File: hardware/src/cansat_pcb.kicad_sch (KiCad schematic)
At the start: 9 parts, among them J1 Servo_motor, J2 Sen057_pressure_sensor, SW1 SPDT_Slide_SMD_6.7x2.6mm, U1 XIAO-nRF52840-Plus-SMD, U2 5V_booster, U3 Hall-effect_sensor, U4 BME280_sensor, U5 Openlog_SDcard

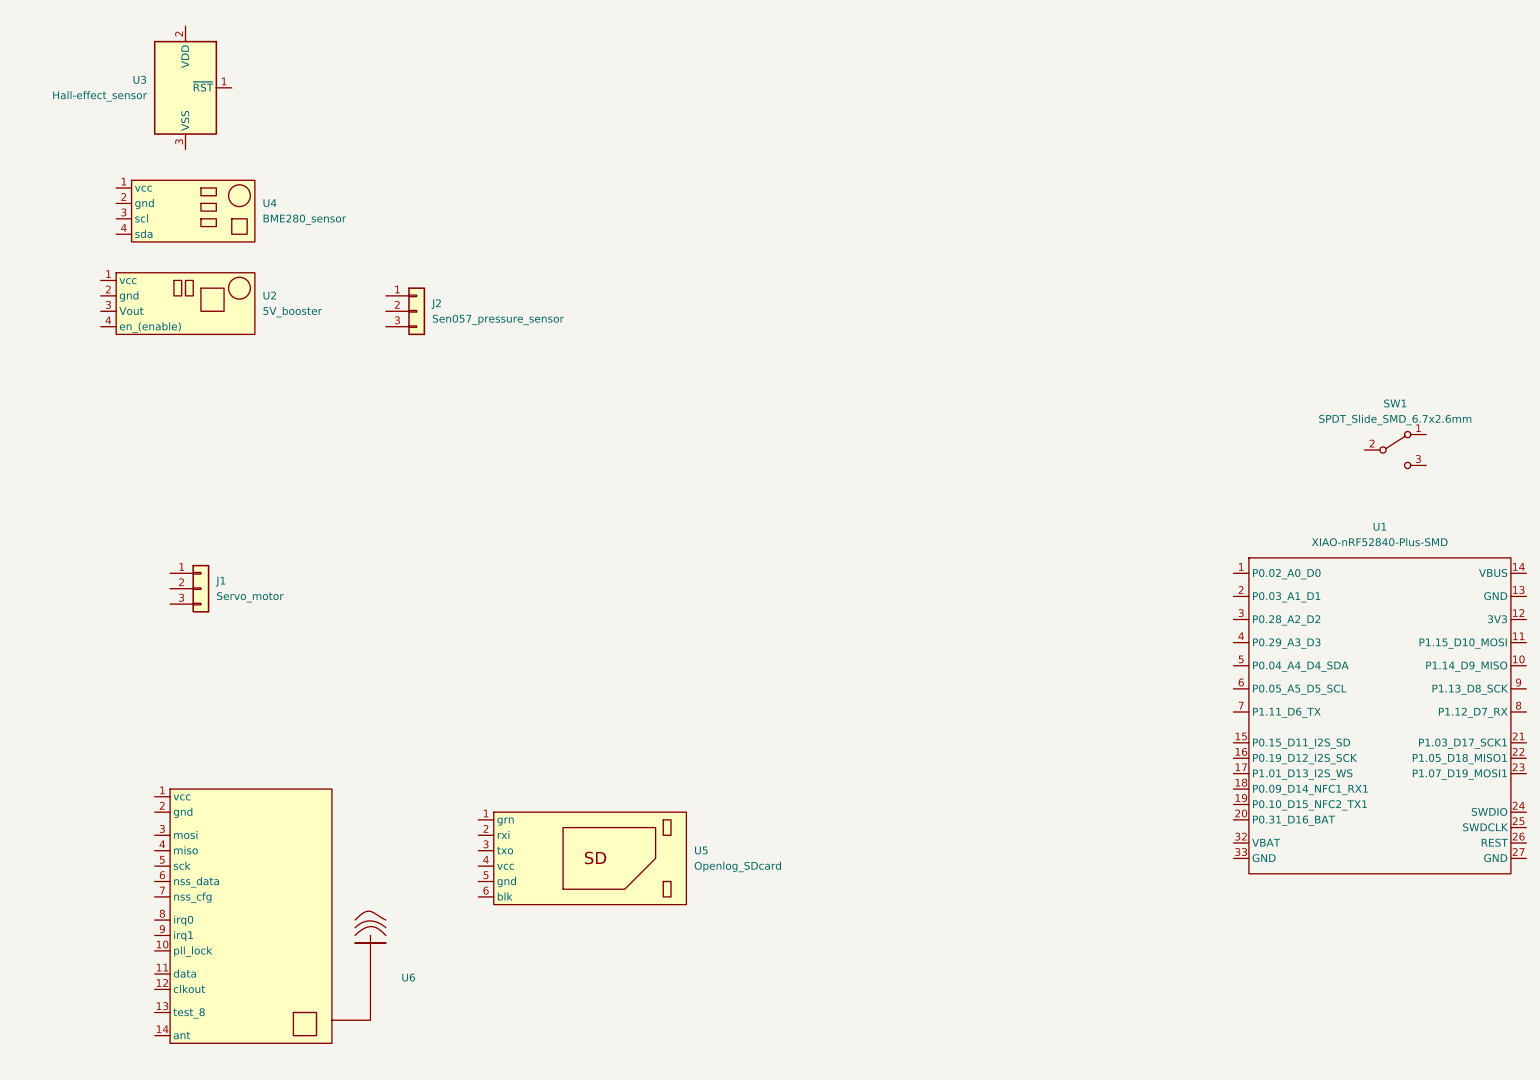
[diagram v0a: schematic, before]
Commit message: feature: pcb started
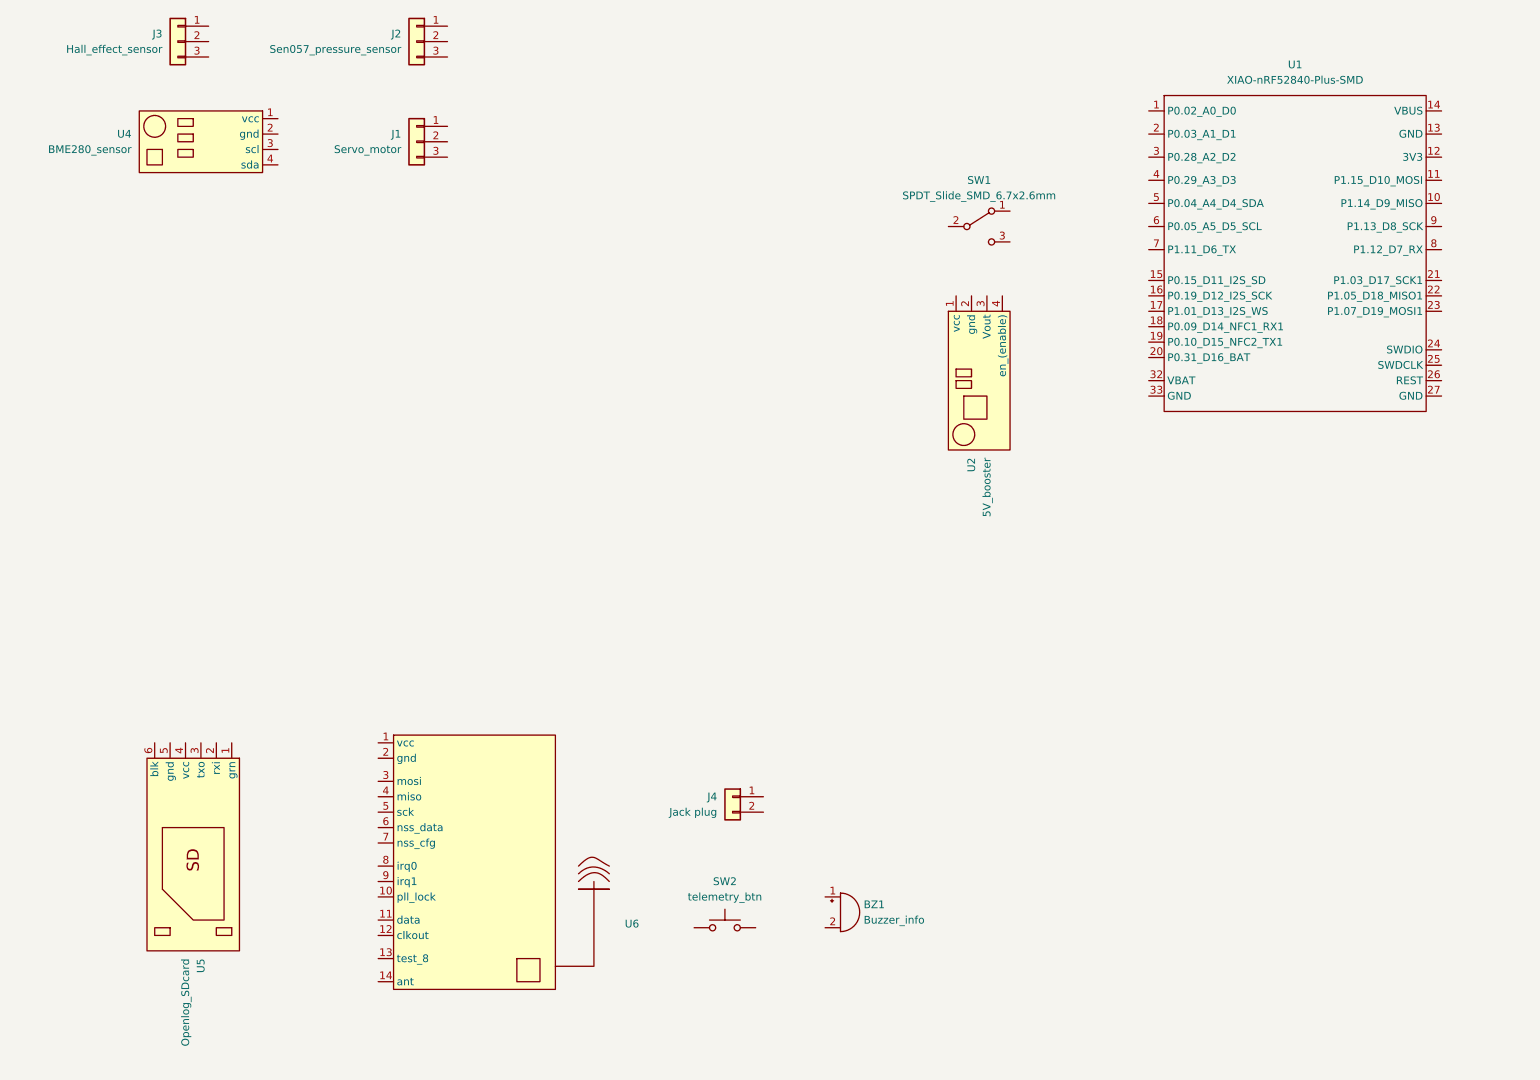
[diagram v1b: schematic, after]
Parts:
- removed U3: Hall-effect_sensor, Package_TO_SOT_THT:TO-92_Inline, symbol Power_Supervisor:MCP120-xxxDxTO
- added BZ1: Buzzer_info, Buzzer_Beeper:Buzzer_12x9.5RM7.6, symbol Device:Buzzer
- added J3: Hall_effect_sensor, Connector_PinHeader_2.54mm:PinHeader_1x03_P2.54mm_Vertical, symbol Connector_Generic:Conn_01x03
- added J4: Jack plug, Connector_PinHeader_1.00mm:PinHeader_1x02_P1.00mm_Horizontal, symbol Connector_Generic:Conn_01x02
- added SW2: telemetry_btn, craby's_library:SW_BUTT-2, symbol Switch:SW_MEC_5G
- SW1: footprint PCM_SparkFun-Switch:Slide_SPST_SMD_6.7x2.6mm -> Button_Switch_SMD:SW_SPDT_CK_JS102011SAQN
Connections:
- new net: SW2.1 (A), SW2.2 (A)
- new net: SW2.3 (B), SW2.4 (B)
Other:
- moved on the sheet: J1, J2, SW1, U1, U2, U4, U5, U6
